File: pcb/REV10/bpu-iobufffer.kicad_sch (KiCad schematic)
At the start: 37 parts, among them J301 Conn_01x10, J302 Conn_01x09, U301 74LVC1T45, U302 74LVC1T45, U303 74LVC1T45, U304 74LVC1T45, U305 74LVC1T45, U306 74LVC1T45, U307 74LVC1T45, U308 74LVC1T45

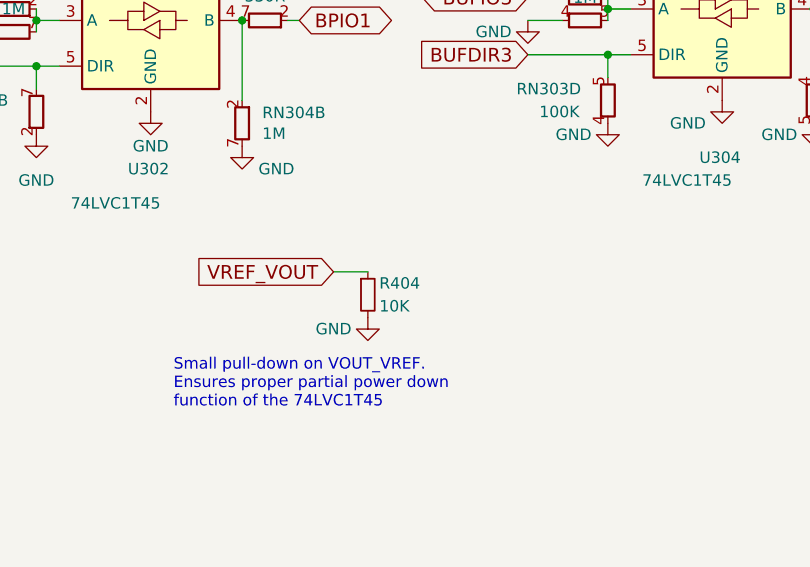
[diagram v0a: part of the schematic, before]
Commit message: making chris branch
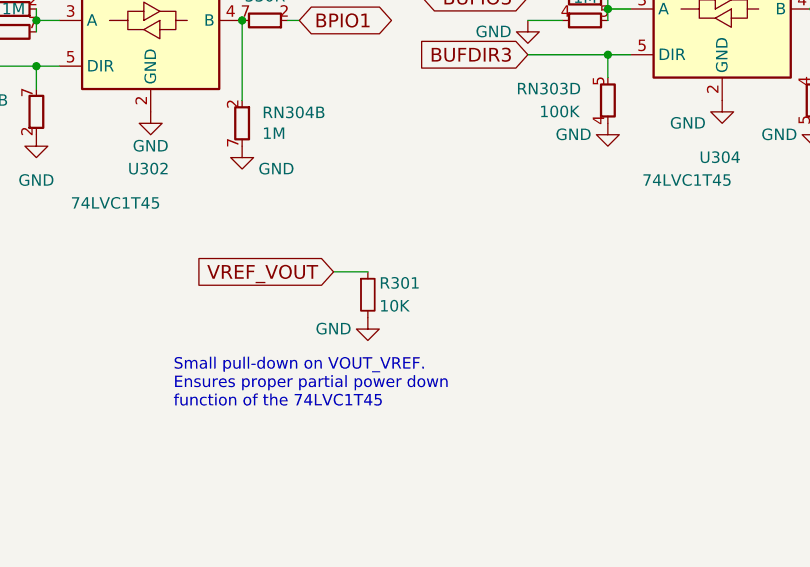
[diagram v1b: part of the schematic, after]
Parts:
- renumbered R404 to R301

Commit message: clean up directory names
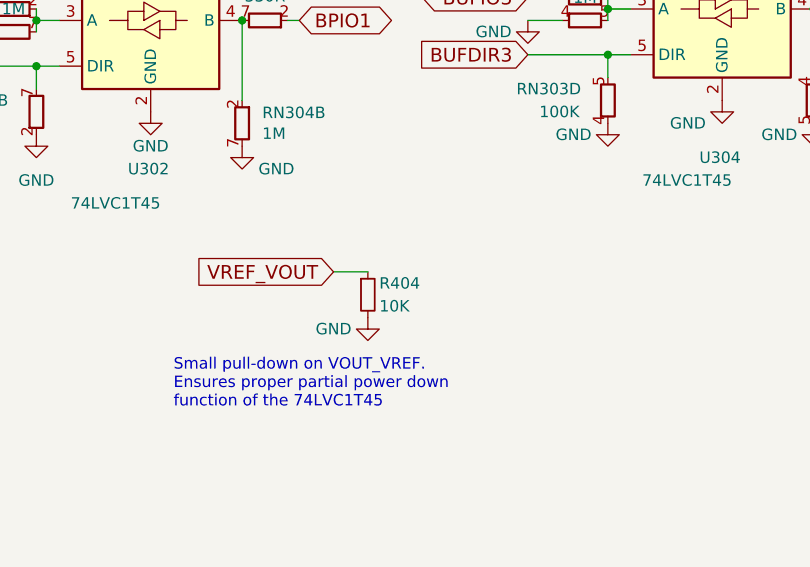
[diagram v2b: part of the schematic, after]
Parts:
- renumbered R301 to R404
